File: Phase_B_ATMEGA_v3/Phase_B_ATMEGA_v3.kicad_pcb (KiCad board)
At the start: 2 copper layers, 49 parts, among them J1 AVR-ISP-6, J2 USB_B_Mini, J3 ESP_Conn, U1 CA56-12EWA, U2 74HC595, U3 ATmega32U4-A, U4 USBLC6-2SC6, U5 LP2985-3.3, Y1 16MHz

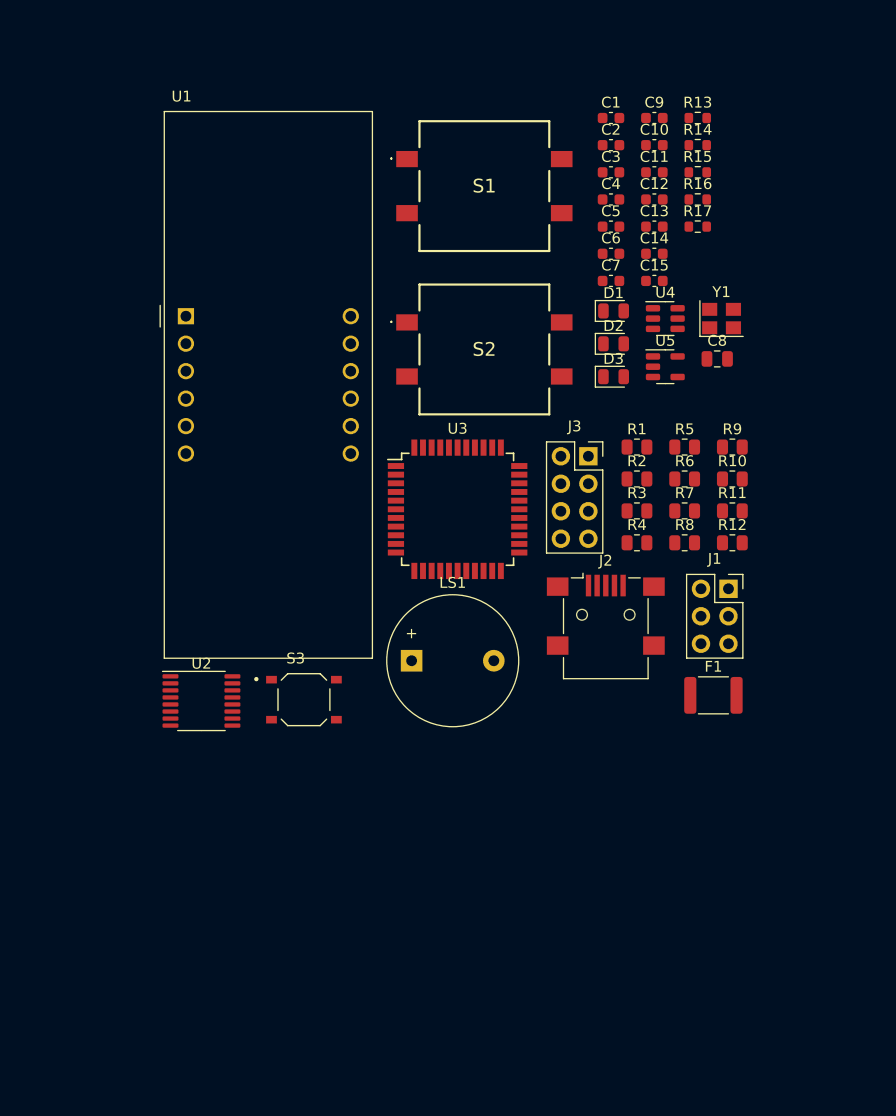
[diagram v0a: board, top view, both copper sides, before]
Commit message: 1
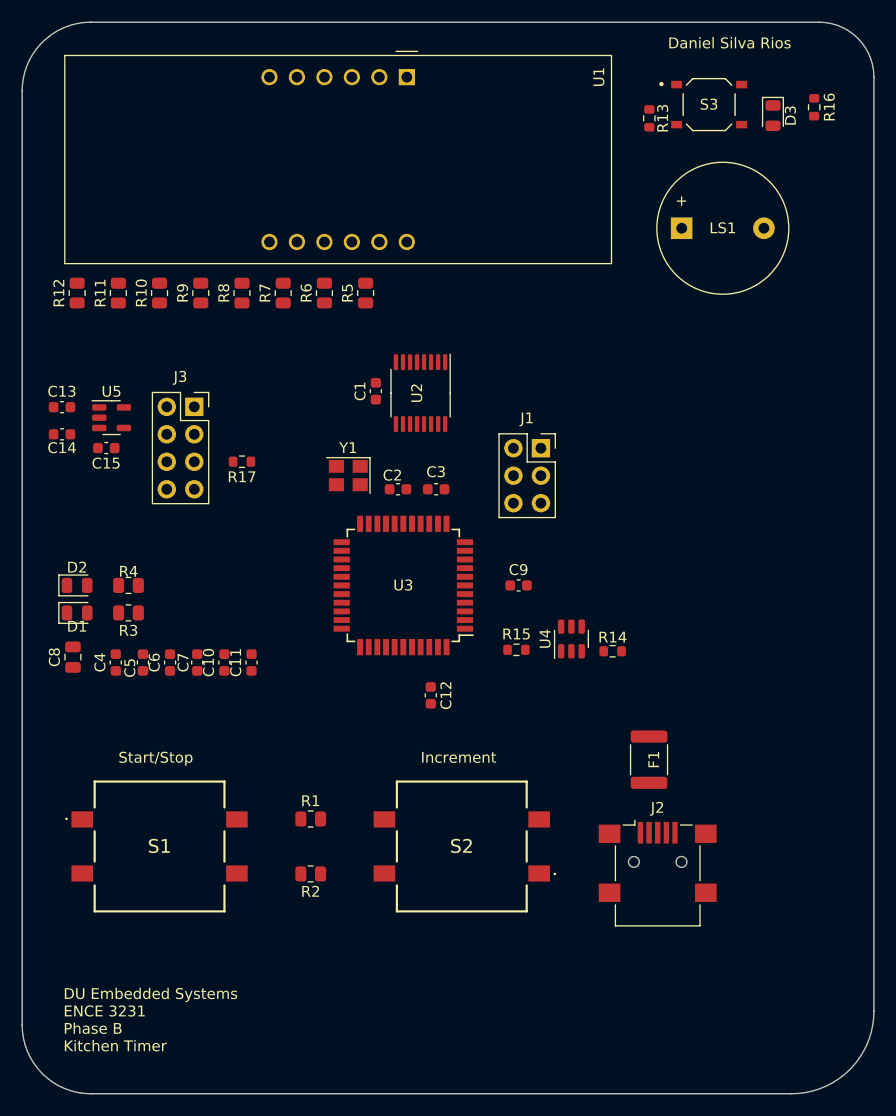
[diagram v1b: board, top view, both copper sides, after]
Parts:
- moved S1 68.0 mm to (120.7, 130.8)
- moved S3 66.5 mm to (171.4, 62.2)
- moved C8 65.6 mm to (112.6, 113.3), turned to 90 degrees
- moved R12 64.8 mm to (113.0, 79.7), turned to 90 degrees
- moved C4 62.7 mm to (116.6, 113.8), turned to 90 degrees
- moved C10 62.2 mm to (126.6, 113.8), turned to 90 degrees
- moved R11 60.2 mm to (116.8, 79.7), turned to 90 degrees
- moved C5 59.1 mm to (119.1, 113.8), turned to 90 degrees
- moved C11 58.7 mm to (129.2, 113.8), turned to 90 degrees
- moved C13 57.2 mm to (111.6, 90.2)
- moved C14 57.2 mm to (111.6, 92.7)
- moved D1 56.9 mm to (113.0, 109.2)
- moved R10 55.7 mm to (120.7, 79.7), turned to 90 degrees
- moved C6 55.6 mm to (121.6, 113.8), turned to 90 degrees
- moved D2 54.4 mm to (113.0, 106.7)
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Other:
- board outline added: 78.7 x 99.1 mm
- board text added: "DU Embedded Systems ENCE 3231 Phase B Kitchen Timer"
- board text added: "Daniel Silva Rios"
- board text added: "Increment"
- board text added: "Start/Stop"
